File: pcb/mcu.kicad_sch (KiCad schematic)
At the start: 38 parts, among them J1 XF2M-1415-1A, SW1 EVQ-Q2B02W, SW2 EVQ-Q2B02W, U1 ESP32-S3-WROOM-1-N8R2

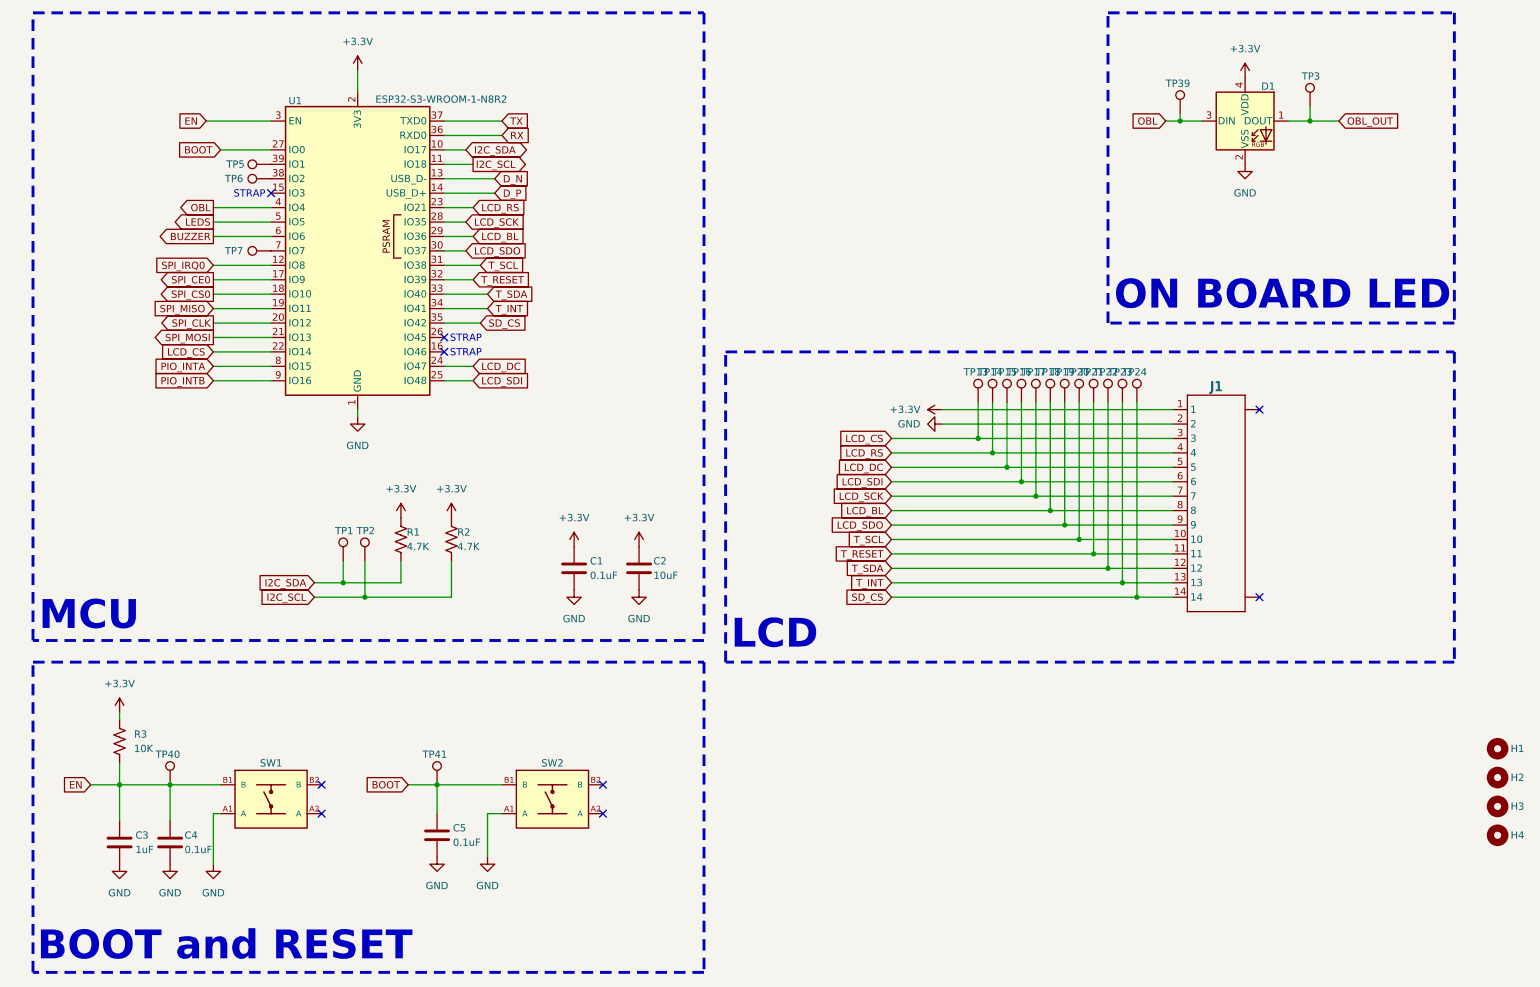
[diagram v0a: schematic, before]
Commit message: Adjusting for consistency
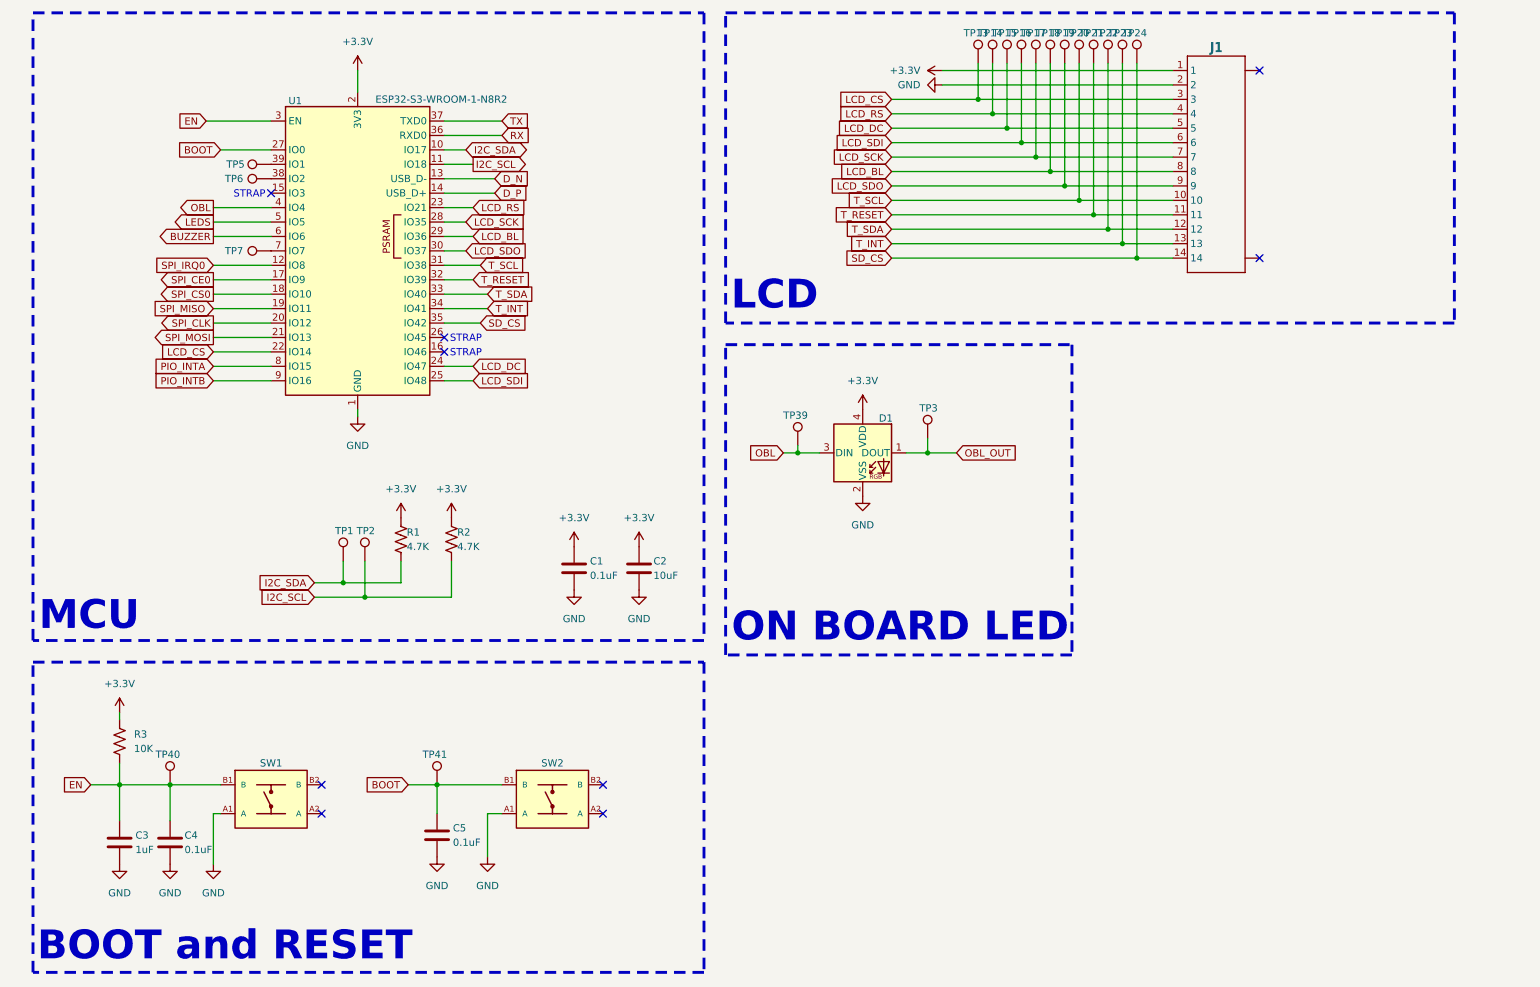
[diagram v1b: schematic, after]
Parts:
- removed H1, H2, H3, H4: ~, CRGM Mechanical:MountingHole_3.2mm_M3_Pad_Via, symbol Mechanical:MountingHole
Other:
- title: Hub Hardware -> Aquarius Hub
- moved on the sheet: D1, J1, TP13, TP14, TP15, TP16, TP17, TP18, TP19, TP20, TP21, TP22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
